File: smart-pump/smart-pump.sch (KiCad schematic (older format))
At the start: 21 parts, among them J1 Screw_Terminal_01x04, Q1 BC337, Q2 IRF5305, SW1 SW_SPST, U1 AMS1117-5.0, U2 Arduino_Pro_Mini

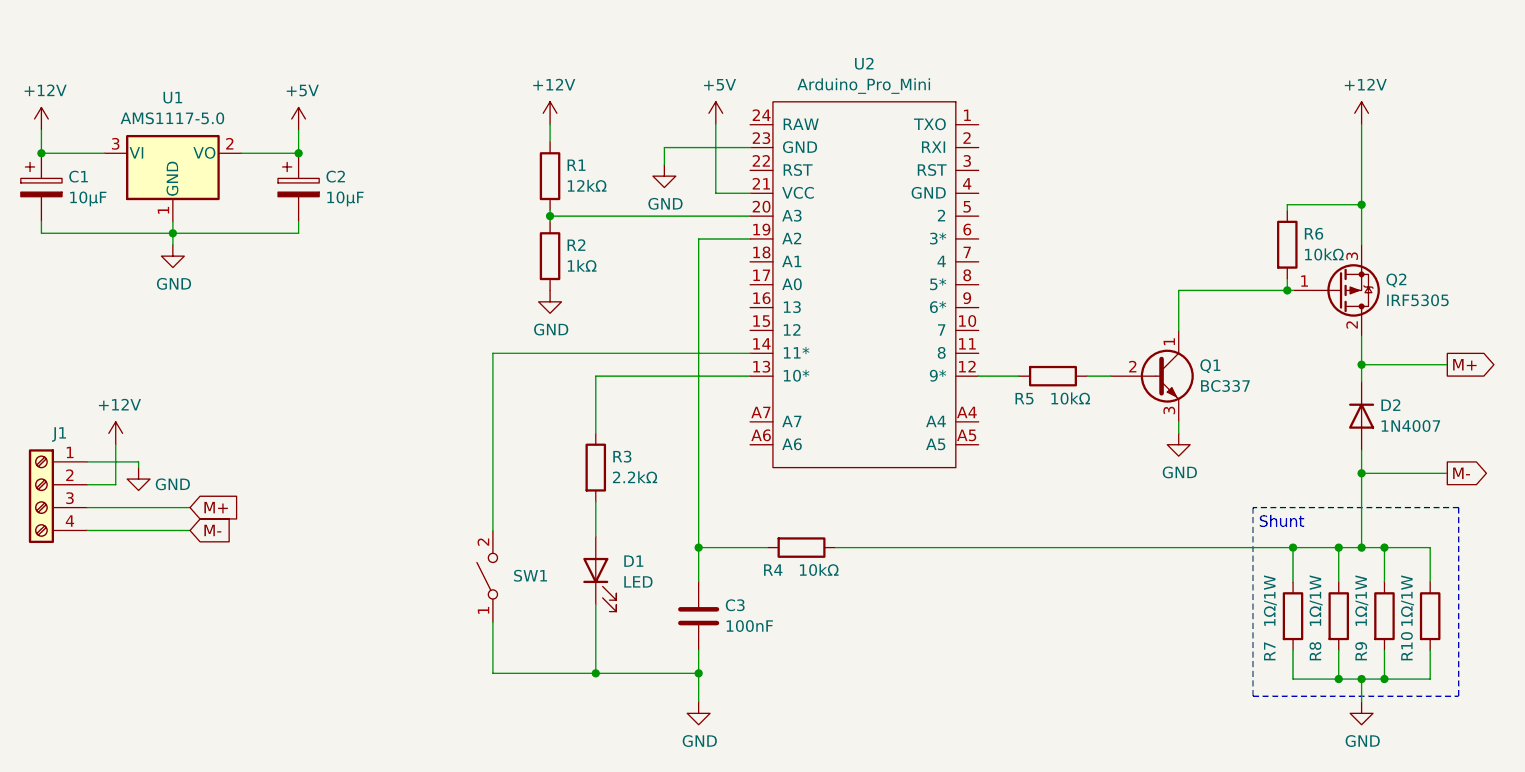
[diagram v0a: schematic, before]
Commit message: Updated smart pump
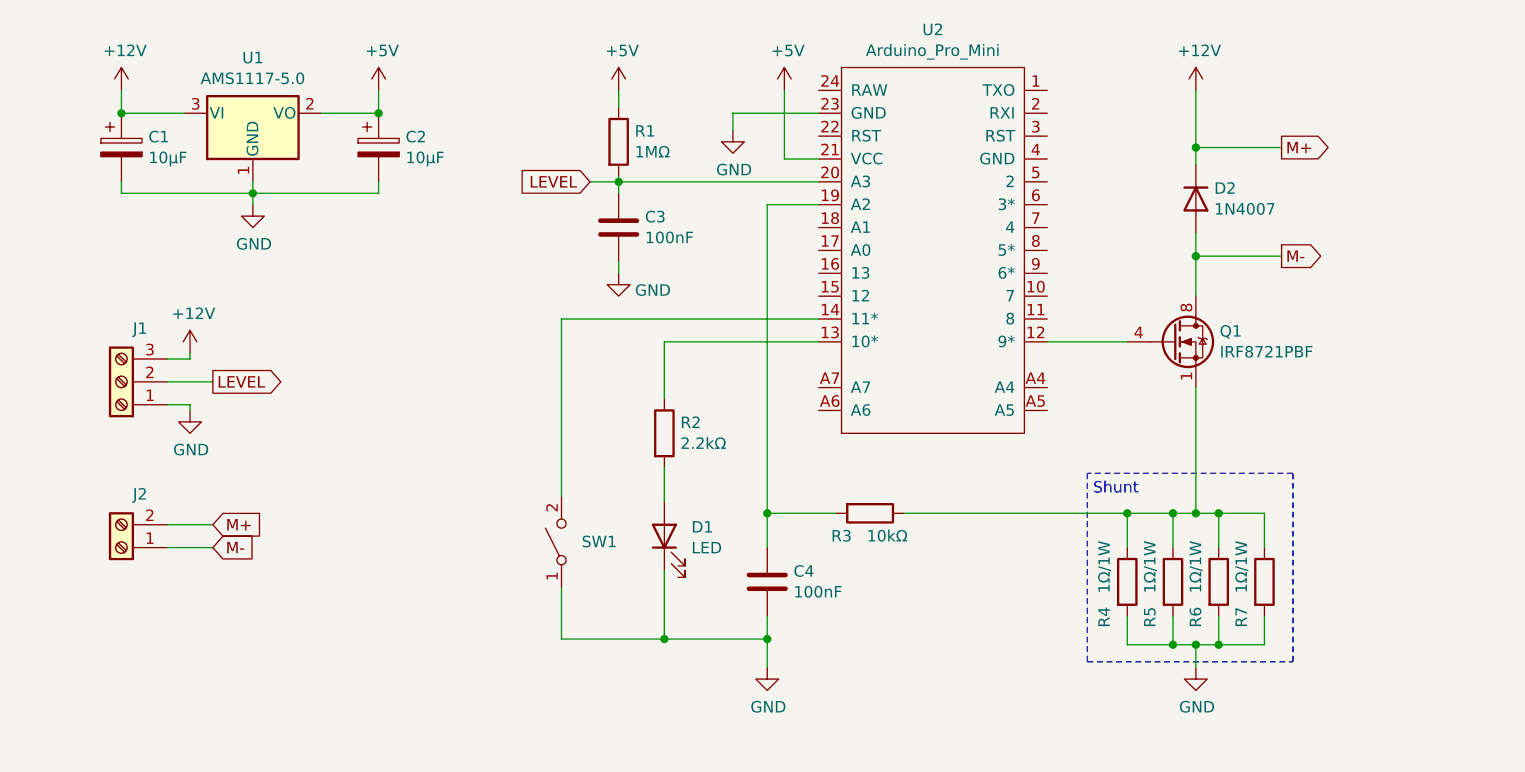
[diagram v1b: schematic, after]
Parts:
- removed J1: Screw_Terminal_01x04, symbol Connector:Screw_Terminal_01x04
- removed Q1: BC337, Package_TO_SOT_THT:TO-92_Inline, symbol Transistor_BJT:BC337
- removed Q2: IRF5305, symbol Device:Q_PMOS_GDS
- removed R2: 1kΩ, symbol Device:R
- removed R5, R6: 10kΩ, symbol Device:R
- added C3: 100nF, symbol Device:C
- added J1: Screw_Terminal_01x03, symbol Connector:Screw_Terminal_01x03
- added J2: Screw_Terminal_01x02, symbol Connector:Screw_Terminal_01x02
- added Q1: IRF8721PBF, Package_SO:SOIC-8_3.9x4.9mm_P1.27mm, symbol Transistor_FET:IRF8721PBF-1
- R1: value 12kΩ -> 1MΩ
- renumbered C3 to C4, R3 to R2, R4 to R3, R7 to R4, R8 to R5, R9 to R6, R10 to R7
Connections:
- net M+ is gone; now on net +12V: D2.1 (K)
- net +12V: now also J1.3 (Pin_3), J2.2 (Pin_2); no longer R1.1
- net +5V: now also R1.1
- net GND: now also C3.2, J1.1 (Pin_1)
- net M-: now also J2.1 (Pin_1), Q1.5 (D), Q1.6 (D), Q1.7 (D), Q1.8 (D); no longer R3.1, R4.1, R5.1, R6.1, R7.1
- net at U2.12 (9*): now also Q1.4 (G)
- net LEVEL: now reaches R1.2, U2.20 (A3)
- net LEVEL: now also C3.1, J1.2 (Pin_2)
- new net: Q1.1 (S), Q1.2 (S), Q1.3 (S), R3.1, R4.1, R5.1, R6.1, R7.1
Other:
- moved on the sheet: C1, C2, C4, D1, D2, R1, R2, R3, R4, R5, R6, R7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
